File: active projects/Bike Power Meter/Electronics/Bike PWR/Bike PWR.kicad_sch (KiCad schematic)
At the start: 26 parts, among them J1 Batt Holder, J3 Analyzer / Flasher, J4 Bridge, U1 LSM6DSLTR, U3 ScioSense PS09

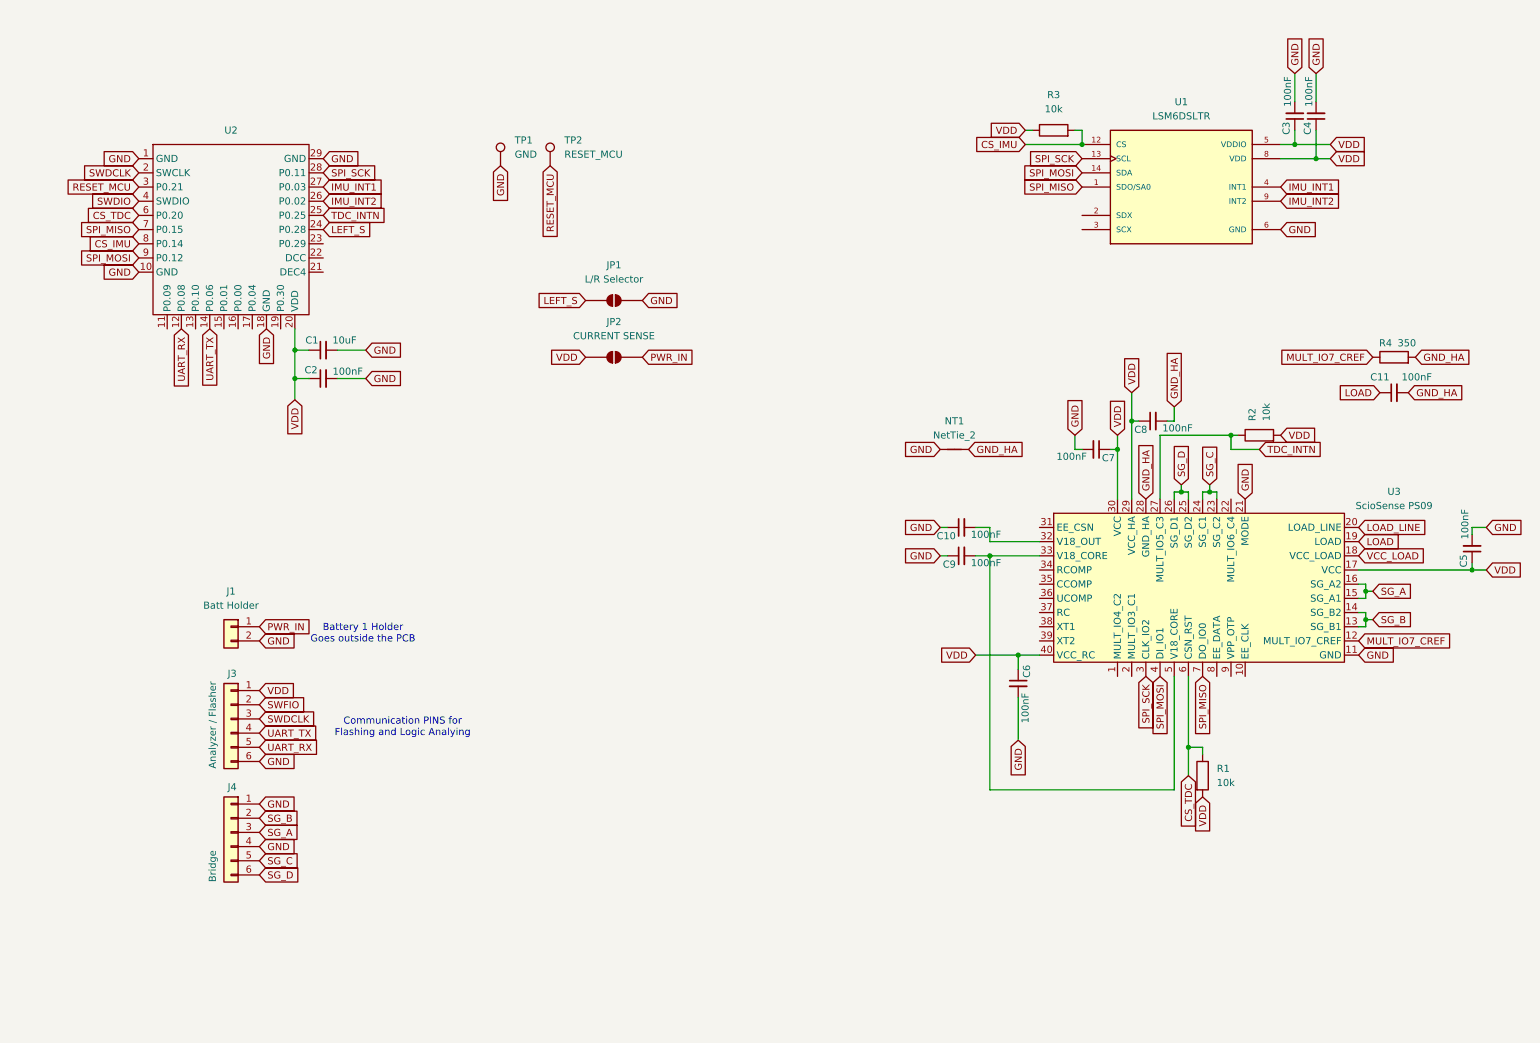
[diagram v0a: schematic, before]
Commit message: Daily update: 2026-08-18 17:32:45
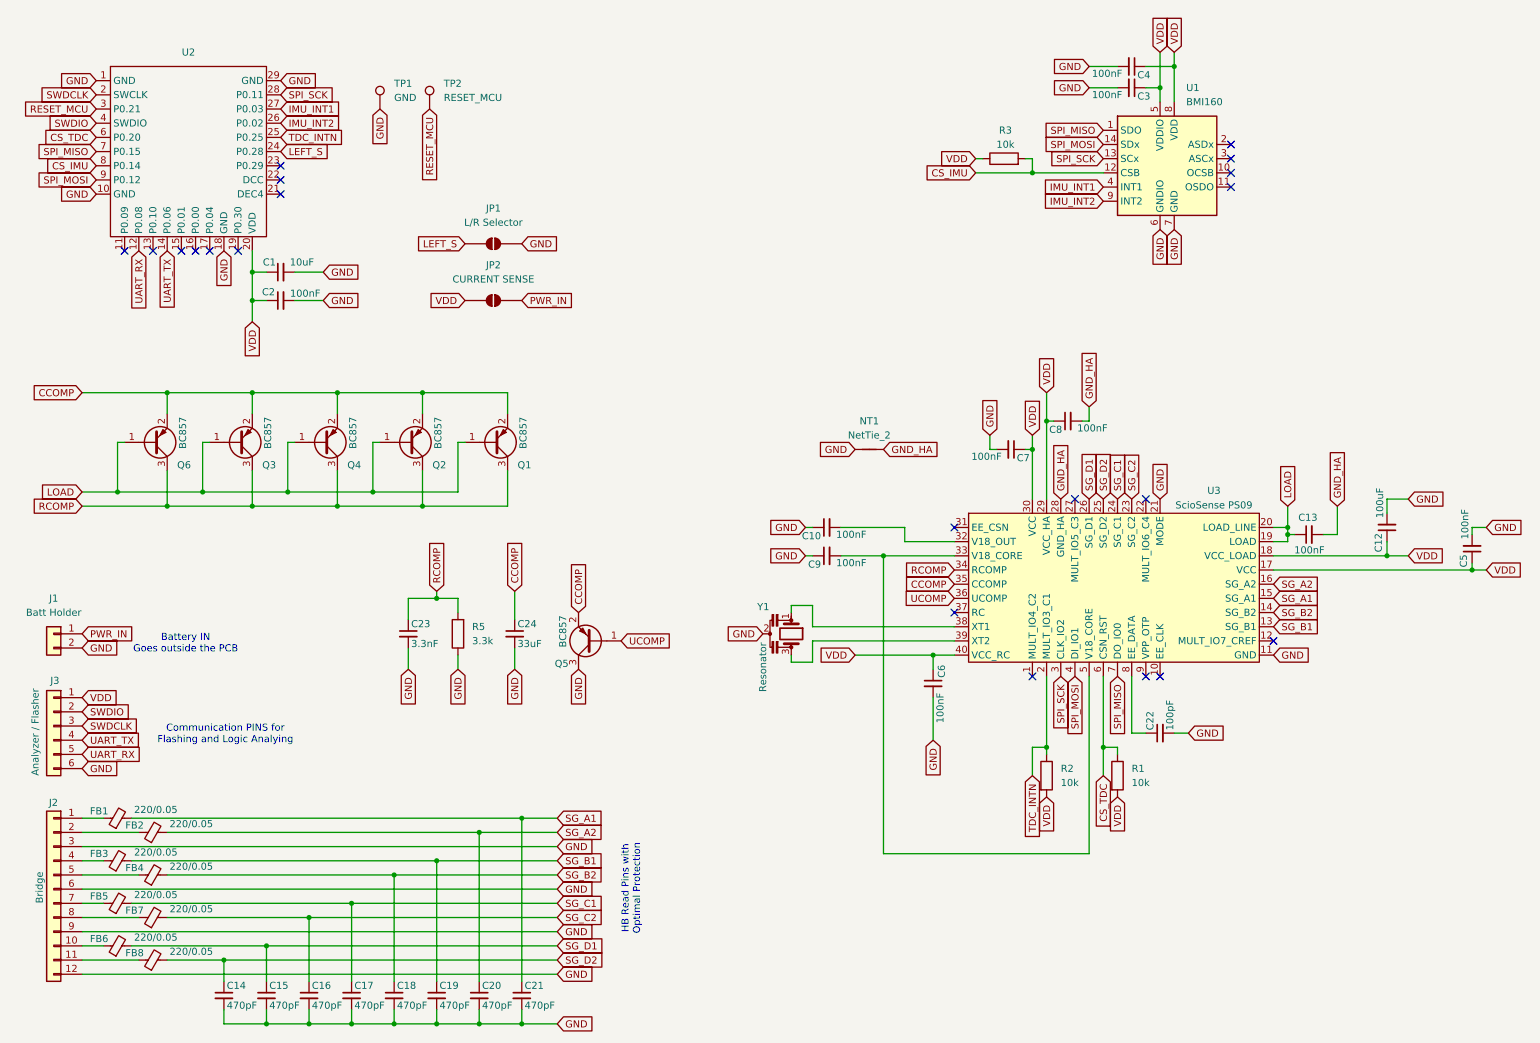
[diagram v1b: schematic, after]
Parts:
- removed C11: 100nF, Capacitor_SMD:C_0201_0603Metric_Pad0.64x0.40mm_HandSolder, symbol Device:C_Small
- removed J4: Bridge, Connector_PinHeader_2.54mm:PinHeader_1x06_P2.54mm_Vertical, symbol Connector_Generic:Conn_01x06
- removed R4: 350, Resistor_SMD:R_0201_0603Metric_Pad0.64x0.40mm_HandSolder, symbol Device:R
- removed U1: LSM6DSLTR, Package_LGA:Bosch_LGA-14_3x2.5mm_P0.5mm, symbol LSM6DSLTR:LSM6DSLTR
- added C12: 100uF, Capacitor_SMD:C_0201_0603Metric_Pad0.64x0.40mm_HandSolder, symbol Device:C_Small
- added C13: 100nF, Capacitor_SMD:C_0201_0603Metric_Pad0.64x0.40mm_HandSolder, symbol Device:C_Small
- added C14, C15, C16, C17, C18, C19, C20, C21: 470pF, Capacitor_SMD:C_0201_0603Metric_Pad0.64x0.40mm_HandSolder, symbol Device:C_Small
- added C22: 100pF, Capacitor_SMD:C_0201_0603Metric_Pad0.64x0.40mm_HandSolder, symbol Device:C_Small
- added C23: 3.3nF, Capacitor_SMD:C_0201_0603Metric_Pad0.64x0.40mm_HandSolder, symbol Device:C_Small
- added C24: 33uF, Capacitor_SMD:C_0201_0603Metric_Pad0.64x0.40mm_HandSolder, symbol Device:C_Small
- added FB1, FB2, FB3, FB4, FB5, FB6, FB7, FB8: 220/0.05, Inductor_SMD:L_0201_0603Metric_Pad0.64x0.40mm_HandSolder, symbol Device:FerriteBead_Small
- added J2: Bridge, Connector_PinHeader_2.54mm:PinHeader_2x06_P2.54mm_Vertical, symbol Connector_Generic:Conn_01x12
- added Q1, Q2, Q3, Q4, Q5, Q6: BC857, Package_TO_SOT_SMD:SOT-23, symbol Transistor_BJT:BC857
- added R5: 3.3k, Resistor_SMD:R_0201_0603Metric_Pad0.64x0.40mm_HandSolder, symbol Device:R
- added U1: BMI160, Package_LGA:Bosch_LGA-14_3x2.5mm_P0.5mm, symbol Sensor_Motion:BMI160
- added Y1: Resonator, bike:OSC_CSTCR4M00G53-R0, symbol Device:Resonator
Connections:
- net LOAD_LINE is gone; now on net LOAD: U3.20 (LOAD_LINE)
- net SWFIO is gone; now on net SWDIO: J3.2 (Pin_2)
- net VCC_LOAD is gone; now on net VDD: U3.18 (VCC_LOAD)
- net CS_IMU: now also U1.12 (CSB)
- net GND: now also C12.2, C14.2, C15.2, C16.2, C17.2, C18.2, C19.2, C20.2, C21.2, C22.2, C23.2, C24.2, J2.12 (Pin_12), J2.3 (Pin_3), J2.6 (Pin_6), J2.9 (Pin_9), Q5.3 (C), R5.1, U1.6 (GNDIO), U1.7 (GND), Y1.2
- net GND_HA: now also C13.2
- net IMU_INT1: now also U1.4 (INT1)
- net IMU_INT2: now also U1.9 (INT2)
- net LOAD: now also C13.1, Q1.1 (B), Q2.1 (B), Q3.1 (B), Q4.1 (B), Q6.1 (B)
- net SPI_MISO: now also U1.1 (SDO)
- net SPI_MOSI: now also U1.14 (SDx)
- net SPI_SCK: now also U1.13 (SCx)
- net TDC_INTN: now also U3.2 (MULT_IO3_C1); no longer U3.27 (MULT_IO5_C3)
- net VDD: now also C12.1, U1.5 (VDDIO), U1.8 (VDD)
- net RCOMP: now reaches U3.34 (RCOMP)
- net RCOMP: now also C23.1, Q1.3 (C), Q2.3 (C), Q3.3 (C), Q4.3 (C), Q6.3 (C), R5.2
- net CCOMP: now reaches U3.35 (CCOMP)
- net CCOMP: now also C24.1, Q1.2 (E), Q2.2 (E), Q3.2 (E), Q4.2 (E), Q5.2 (E), Q6.2 (E)
- net UCOMP: now reaches U3.36 (UCOMP)
- net UCOMP: now also Q5.1 (B)
- net at U3.38 (XT1): now also Y1.1
- net at U3.39 (XT2): now also Y1.3
- net at U3.8 (EE_DATA): now also C22.1
- net MULT_IO7_CREF: no longer names the net of U3.12 (MULT_IO7_CREF)
- net SG_A renamed SG_A1
- net SG_A1: now also C21.1, FB1.2; no longer U3.16 (SG_A2)
- net SG_B renamed SG_B1
- net SG_B1: now also C19.1, FB3.2; no longer U3.14 (SG_B2)
- net SG_C renamed SG_C1
- net SG_C1: now also C17.1, FB5.2; no longer U3.23 (SG_C2)
- net SG_D renamed SG_D1
- net SG_D1: now also C15.1, FB6.2; no longer U3.25 (SG_D2)
- new net: FB6.1, J2.10 (Pin_10)
- new net: FB3.1, J2.4 (Pin_4)
- new net: FB7.1, J2.8 (Pin_8)
- new net: FB4.1, J2.5 (Pin_5)
- new net: FB8.1, J2.11 (Pin_11)
- new net: FB1.1, J2.1 (Pin_1)
- new net: FB2.1, J2.2 (Pin_2)
- new net: FB5.1, J2.7 (Pin_7)
- new net SG_A2: C20.1, FB2.2, U3.16 (SG_A2)
- new net SG_B2: C18.1, FB4.2, U3.14 (SG_B2)
- new net SG_C2: C16.1, FB7.2, U3.23 (SG_C2)
- new net SG_D2: C14.1, FB8.2, U3.25 (SG_D2)
- no-connect marks 0 -> 21
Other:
- note added: "Battery IN Goes outside the PCB"
- note added: "HB Read Pins with Optimal Protection"
- note removed: "Battery 1 Holder Goes outside the PCB"
- moved on the sheet: C1, C10, C2, C3, C4, C6, C7, C8, C9, J1, J3, JP1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
